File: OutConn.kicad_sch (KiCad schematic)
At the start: 4 parts, among them J5 USB_A_Stacked, J6 2041441-1

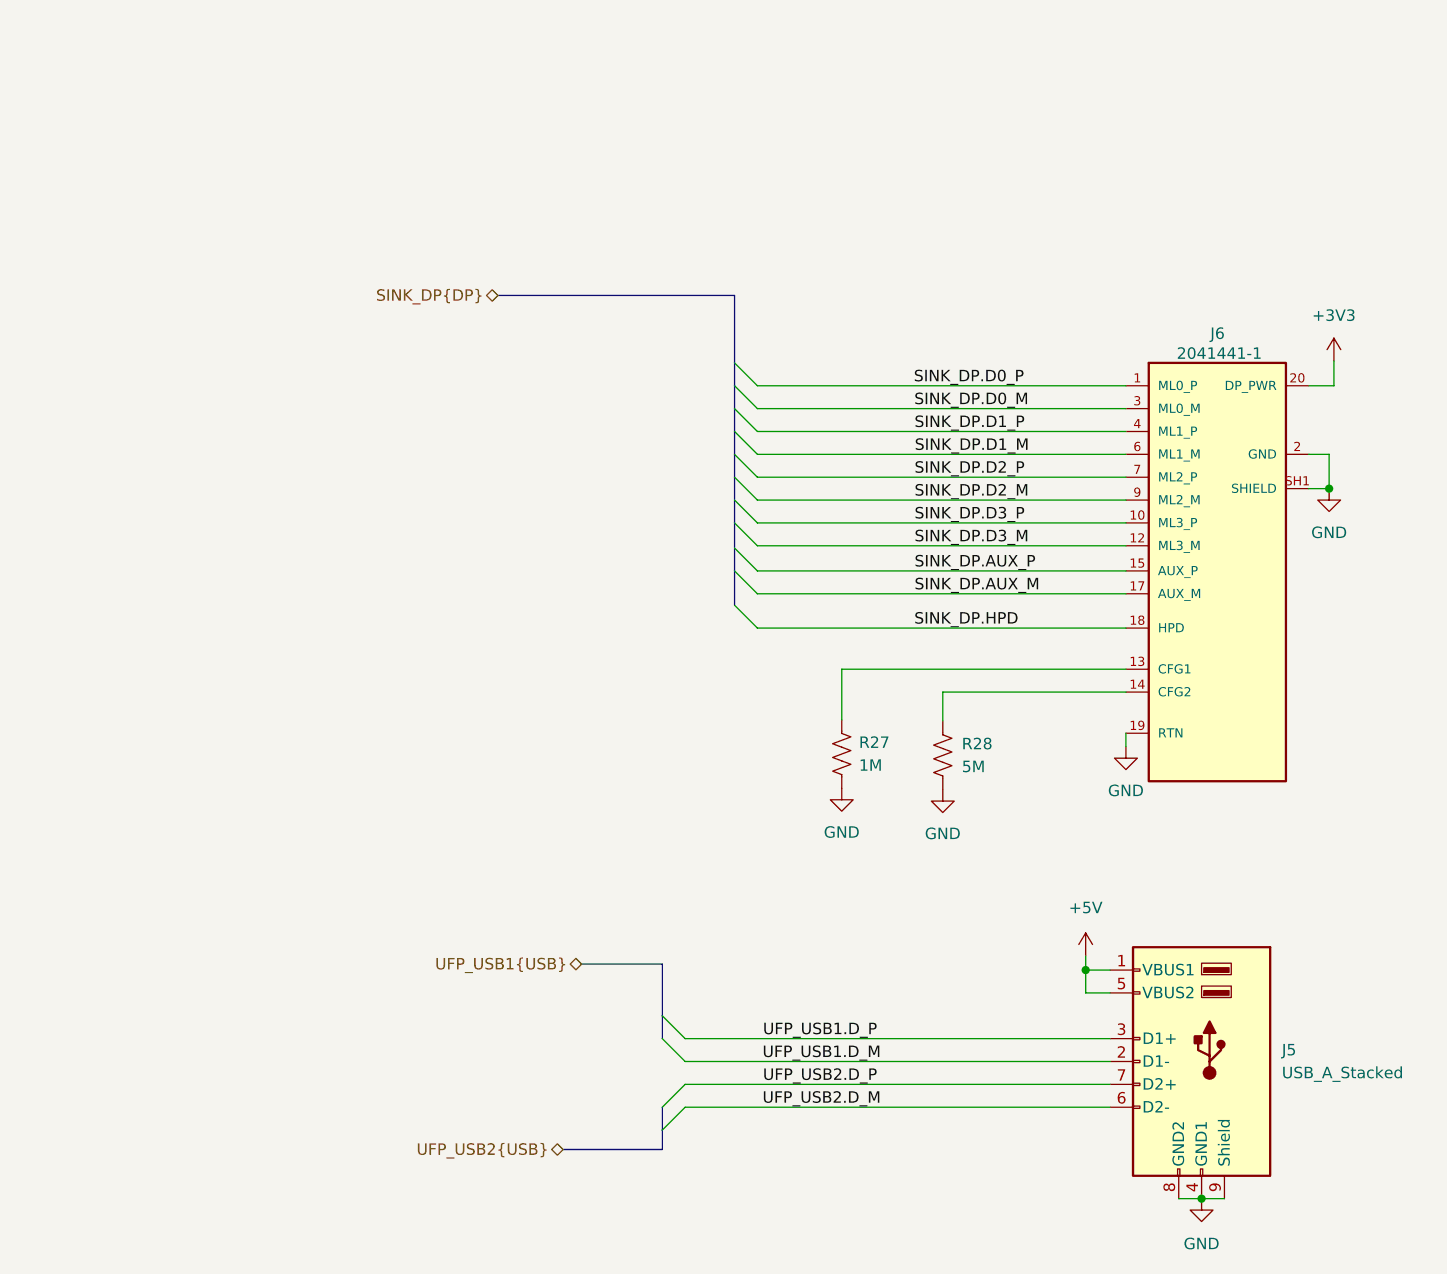
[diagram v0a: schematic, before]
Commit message: Pushing what i have now
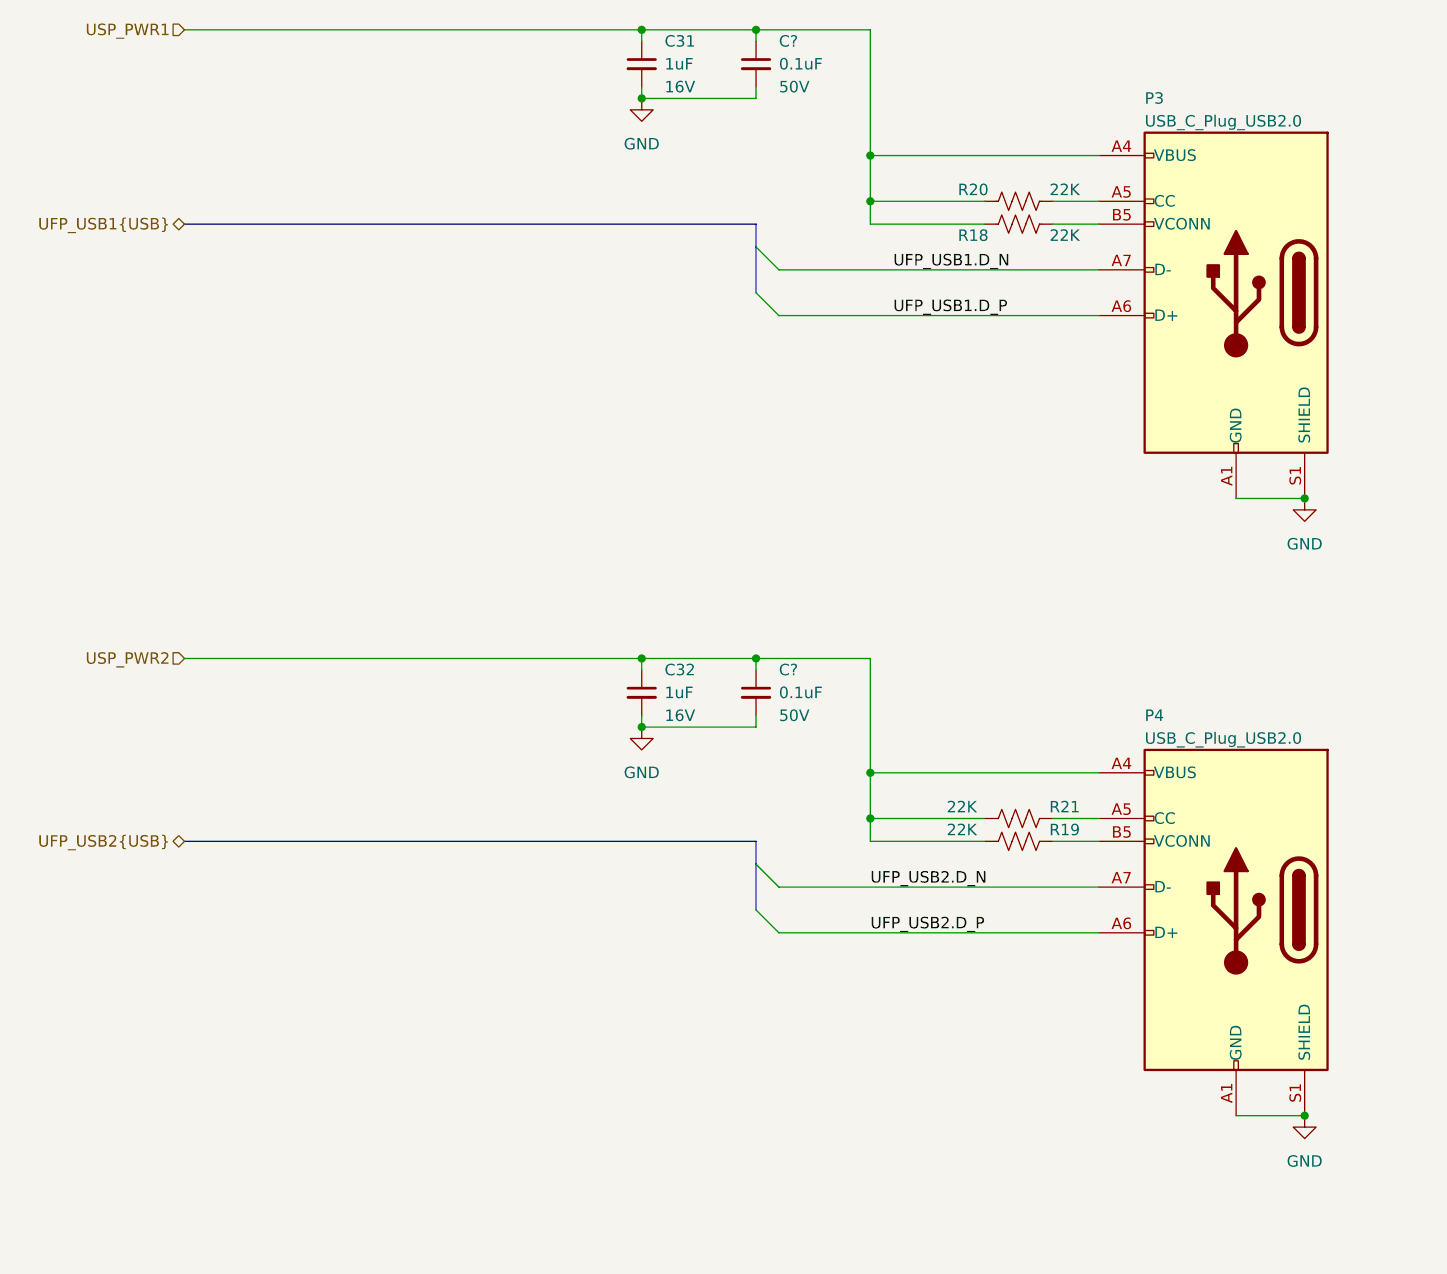
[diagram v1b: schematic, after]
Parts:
- removed J5: USB_A_Stacked, symbol Connector:USB_A_Stacked
- removed J6: 2041441-1, TE_2041441-1, symbol 2041441-1:DP_CONN
- removed R27: 1M, symbol Device:R_US
- removed R28: 5M, symbol Device:R_US
- added C31, C32: ${Capacitance}, Capacitor_SMD:C_0603_1608Metric_Pad1.08x0.95mm_HandSolder, symbol Rockerrobotics:Capacitors/1276-1034-1-ND
- added C? (x2): ${Capacitance}, Capacitor_SMD:C_0603_1608Metric_Pad1.08x0.95mm_HandSolder, symbol Rockerrobotics:Capacitors/1276-1935-1-ND
- added P3, P4: USB_C_Plug_USB2.0, Rockerrobotics:AMPHENOL_12402012E212A, symbol Rockerrobotics:Connectors/664-12402012E212ADKR-ND
- added R18, R19, R20, R21: ${Resistance}, Resistor_SMD:R_0805_2012Metric_Pad1.20x1.40mm_HandSolder, symbol Rockerrobotics:Resistors/13-RC0805FR-1322KLCT-ND
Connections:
- net GND: now also C31.2, C32.2, C?.2, C?.2, P3.A1 (GND), P3.A12 (GND), P3.B1 (GND), P3.B12 (GND), P3.S1 (SHIELD), P4.A1 (GND), P4.A12 (GND), P4.B1 (GND), P4.B12 (GND), P4.S1 (SHIELD)
- net UFP_USB1.D_P: now also P3.A6 (D+)
- net UFP_USB2.D_P: now also P4.A6 (D+)
- new net: P4.B5 (VCONN), R19.2
- new net: P3.B5 (VCONN), R18.2
- new net: P4.A5 (CC), R21.2
- new net: P3.A5 (CC), R20.2
- new net UFP_USB1.D_N: P3.A7 (D-)
- new net UFP_USB2.D_N: P4.A7 (D-)
- new net USP_PWR1: C31.1, C?.1, P3.A4 (VBUS), P3.A9 (VBUS), P3.B4 (VBUS), P3.B9 (VBUS), R18.1, R20.1
- new net USP_PWR2: C32.1, C?.1, P4.A4 (VBUS), P4.A9 (VBUS), P4.B4 (VBUS), P4.B9 (VBUS), R19.1, R21.1
